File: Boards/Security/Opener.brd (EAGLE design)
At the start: 59.4 x 51.8 mm, 43 parts, among them J1 AVR_SPI_PRG_6PTH

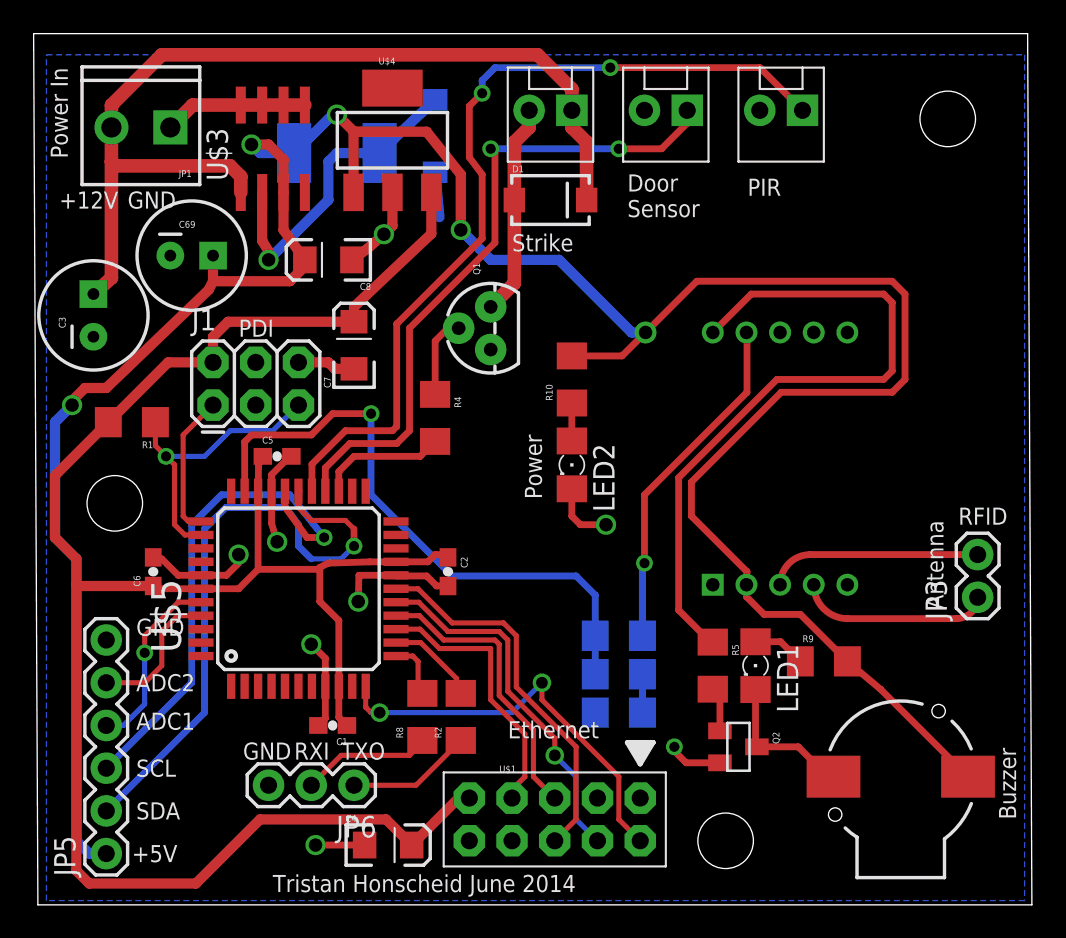
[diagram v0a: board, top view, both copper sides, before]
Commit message: Prepared board for production, last minute error checks and rotations
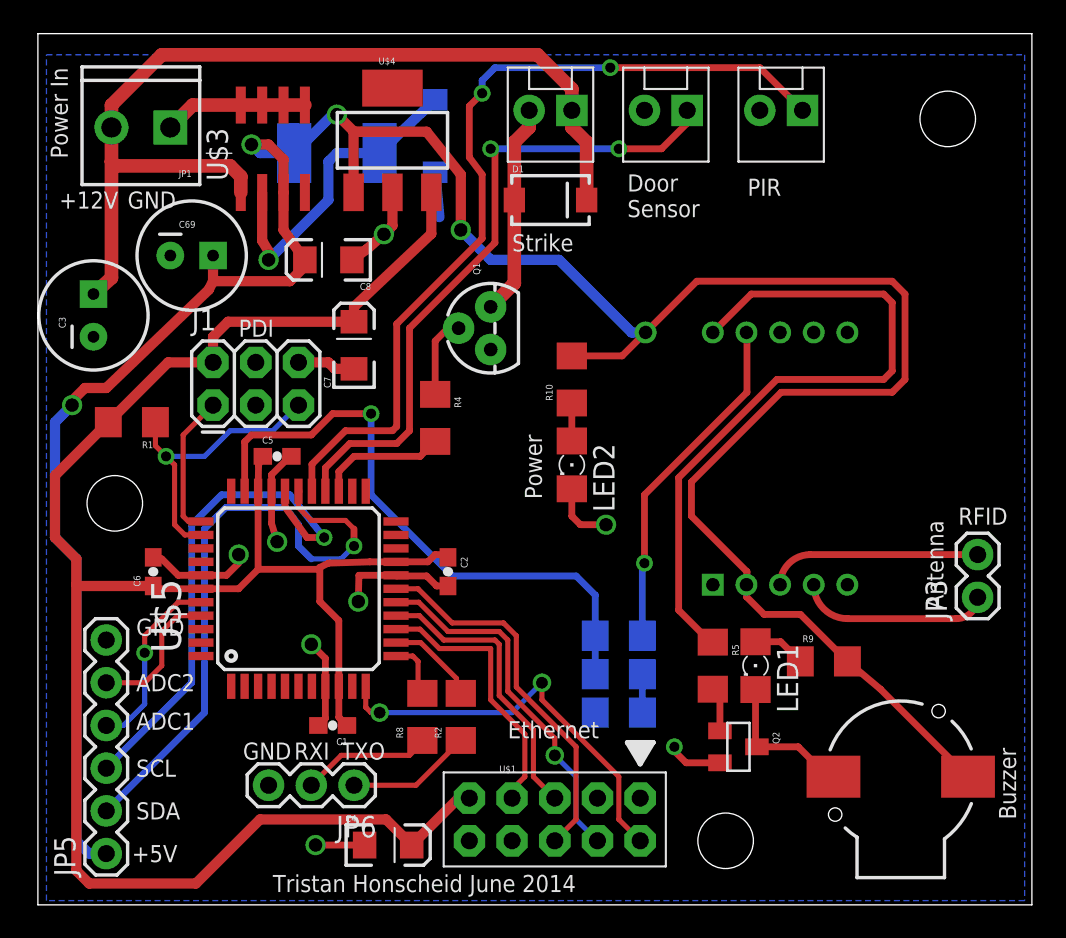
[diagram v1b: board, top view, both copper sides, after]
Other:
- board size 59.4 x 51.8 mm -> 59.1 x 51.8 mm
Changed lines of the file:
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@@
 <?xml version="1.0" encoding="utf-8"?>
 <!DOCTYPE eagle SYSTEM "eagle.dtd">
-<eagle version="7.1.0">
+<eagle version="6.6.0">
 <drawing>
 <settings>
@@
 <plain>
 <wire x1="0" y1="0" x2="59.106" y2="0" width="0" layer="20"/>
-<wire x1="59.106" y1="0" x2="58.852" y2="51.806" width="0" layer="20"/>
-<wire x1="58.852" y1="51.806" x2="-0.254" y2="51.806" width="0" layer="20"/>
-<wire x1="-0.254" y1="51.806" x2="0" y2="0" width="0" layer="20"/>
+<wire x1="59.106" y1="0" x2="59.106" y2="51.806" width="0" layer="20"/>
+<wire x1="59.106" y1="51.806" x2="0" y2="51.806" width="0" layer="20"/>
+<wire x1="0" y1="51.806" x2="0" y2="0" width="0" layer="20"/>
 <text x="35.052" y="40.894" size="1.016" layer="21">Door
 Sensor</text>
@@
 <pass name="Default">
 <param name="RoutingGrid" value="50mil"/>
-<param name="AutoGrid" value="1"/>
-<param name="Efforts" value="0"/>
-<param name="TopRouterVariant" value="1"/>
 <param name="tpViaShape" value="round"/>
 <param name="PrefDir.1" value="|"/>
